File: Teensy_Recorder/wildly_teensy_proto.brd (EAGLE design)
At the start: 60.7 x 77.5 mm, 40 parts, among them J1 61300211121, J2 61300311121, J3 61300311121, T1 BC847BLT1G, T2 BC847BLT1G, T3 BC847BLT1G, T4 BC847BLT1G

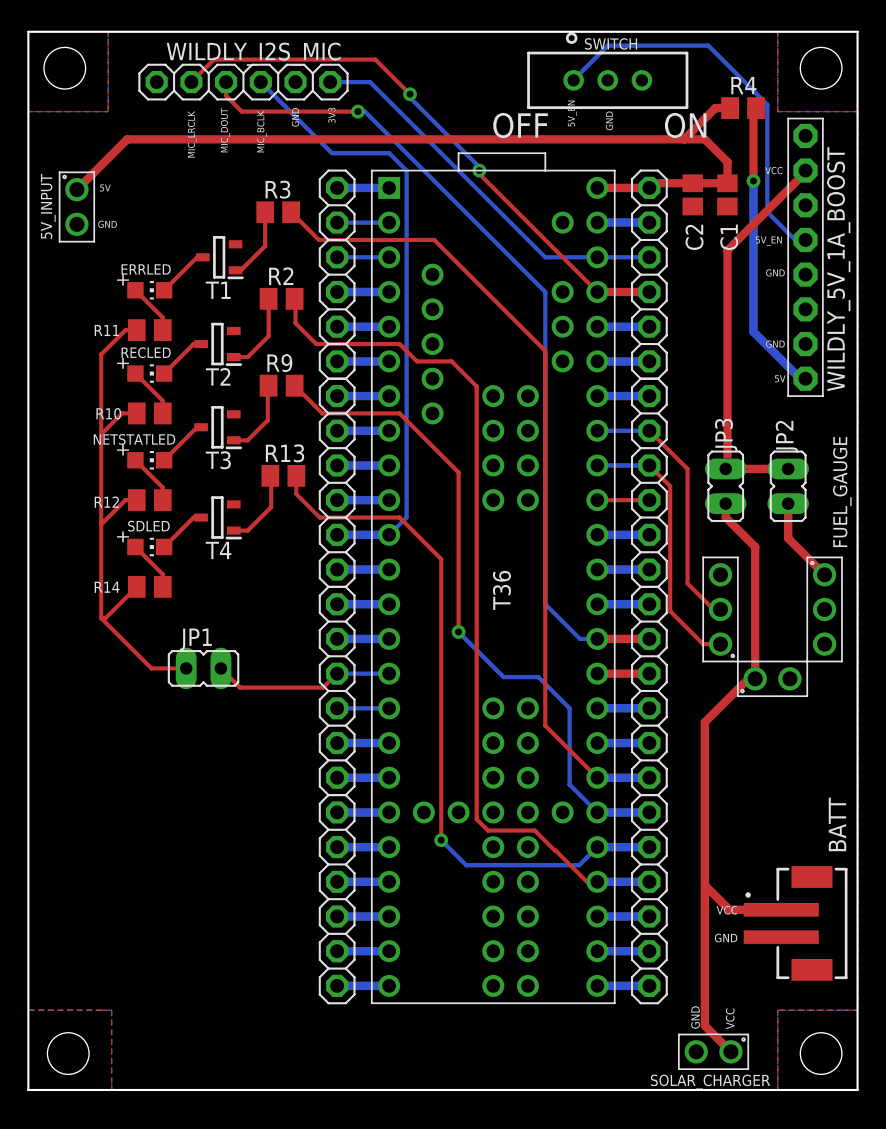
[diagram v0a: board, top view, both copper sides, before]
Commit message: Rework recroder board to be more compact, remove unnecessary components etc
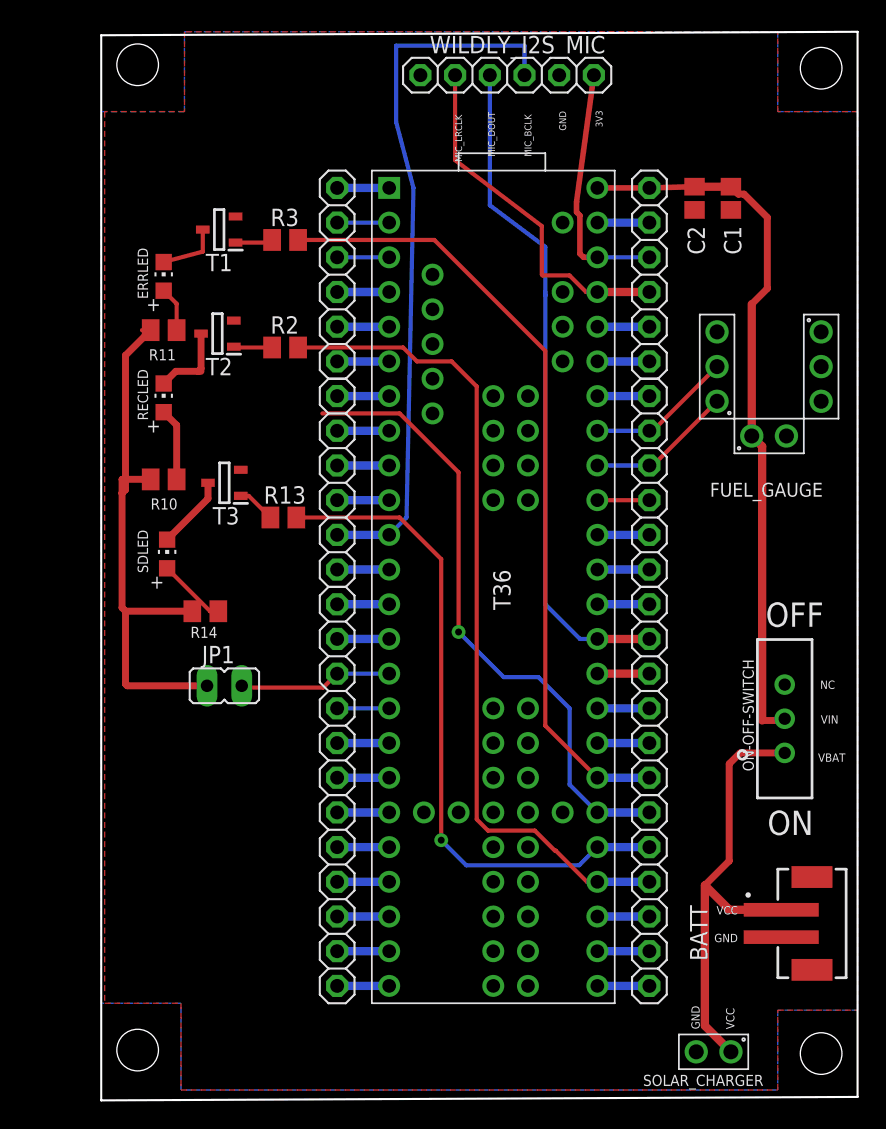
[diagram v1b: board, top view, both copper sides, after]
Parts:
- removed 5V_INPUT: 61300211121, 61300211121:61300211121
- removed JP2, JP3: (no value), jumper:JP1
- removed NETSTATLED: (no value), adafruit:CHIP-LED0805
- removed R12: 870R, adafruit:M0805
- removed R4: 0R, adafruit:M0805
- removed R9: 1.65KR, adafruit:M0805
- removed SWITCH: GSM Power, EG1218:3PIN_SLIDE_SWITCH
- removed T4: BC847BLT1G, BC847BLT1G:SOT96P237X111-3N
- removed WILDLY_5V_1A_BOOST: (no value), adafruit:1X08-BIG
- added ON-OFF-SWITCH: Power, EG1218:3PIN_SLIDE_SWITCH
- moved WILDLY_I2S_MIC 19.3 mm to (35.1, 74.3)
- moved J2 17.8 mm to (50.4, 53.0)
- moved J3 17.8 mm to (58.0, 53.0)
- moved J1 17.8 mm to (54.2, 47.9)
- moved R10 4.93 mm to (9.91, 44.7)
- moved R14 4.44 mm to (13.0, 35.1)
- moved T3 4.10 mm to (14.4, 44.5)
- moved R2 3.57 mm to (18.8, 54.4)
- moved R13 3.05 mm to (18.7, 41.9)
- moved R3 2.09 mm to (18.8, 62.2)
- moved RECLED 2.05 mm to (9.91, 50.7), turned to 0 degrees
- moved T1 2.03 mm to (14.0, 63.0)
- moved JP1 1.98 mm to (14.4, 29.6)
- moved ERRLED 1.44 mm to (9.91, 59.6), turned to 0 degrees
- moved SDLED 1.37 mm to (10.2, 39.2), turned to 0 degrees
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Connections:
- removed net +5V: 5V_INPUT.1, C1.1, C2.1, R4.1, TEENSY_PIN_5.1, U$1.VIN
- removed net 5V_EN: SWITCH.1, WILDLY_5V_1A_BOOST.5
- removed net 5V_SUPPLY: R4.2, WILDLY_5V_1A_BOOST.1
- removed net LB: WILDLY_5V_1A_BOOST.3
- removed net N$12: J3.1, JP2.1
- removed net N$16: NETSTATLED.A, R12.1
- removed net N$5: NETSTATLED.C, T3.3
- removed net N$6: WILDLY_5V_1A_BOOST.6
- removed net N$7: R9.2, T3.1
- removed net VCCIO: JP2.2, JP3.1, WILDLY_5V_1A_BOOST.7
- new net VIN: C1.1, C2.1, J1.1, ON-OFF-SWITCH.2, TEENSY_PIN_5.1, U$1.VIN
- net +3V3: no longer R12.2
- net GND: no longer 5V_INPUT.2, SWITCH.2, T4.2, WILDLY_5V_1A_BOOST.2, WILDLY_5V_1A_BOOST.4
- net N$1: now also T3.3; no longer T4.3
- net N$11: now also T3.1; no longer T4.1
- net NETSTATLED: no longer R9.1
- net VCC: now also ON-OFF-SWITCH.1; no longer J1.1, JP3.2
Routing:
- net +5V: track 65.4 -> 0.00 mm
- net VIN: track 0.00 -> 52.7 mm
- net VCCIO: track 28.8 -> 0.00 mm
- net 5V_EN: track 28.6 -> 0.00 mm
- net 5V_SUPPLY: track 21.7 -> 0.00 mm, vias 1 -> 0
- net VCC: track 50.0 -> 33.3 mm
- net MIC_LRCLK: track 41.7 -> 26.2 mm, vias 2 -> 0
- net MIC_DOUT: track 61.9 -> 49.7 mm, vias 1 -> 0
- net 3V3: track 42.8 -> 30.8 mm
- net FUEL_GAUGE_SDA: track 19.8 -> 10.7 mm
- net FUEL_GAUGE_SCL: track 19.3 -> 10.7 mm
- net MIC_BCLK: track 44.4 -> 51.9 mm
- net N$12: track 6.31 -> 0.00 mm
- net N$7: track 5.66 -> 0.00 mm
- net N$16: track 3.75 -> 0.00 mm
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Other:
- board size 60.7 x 77.5 mm -> 55.4 x 78.2 mm
- board text added: "NC"
- board text added: "VBAT"
- board text added: "VIN"
- board text added: "Wildly_Listen_Recorder_V1"
- board text removed: "5V"
- board text removed: "5V_EN"
- board text removed: "Wildly_Listen_Proto_V1"
